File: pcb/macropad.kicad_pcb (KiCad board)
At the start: 2 copper layers, 135 x 79.3 mm, 36 parts, among them J1 Conn_01x02_Pin, SW1 SW_Push, SW10 SW_Push, SW11 SW_Push, SW12 SW_Push, SW13 SW_Push, SW14 SW_Push, SW15 SW_Push, SW16 SW_Push, SW17 SW_DIP_x01, SW18 SW_Push, SW2 SW_Push, SW3 SW_Push, SW4 SW_Push, SW5 SW_Push, SW6 SW_Push, SW7 SW_Push, SW8 SW_Push, SW9 SW_Push, U2 ProMicro

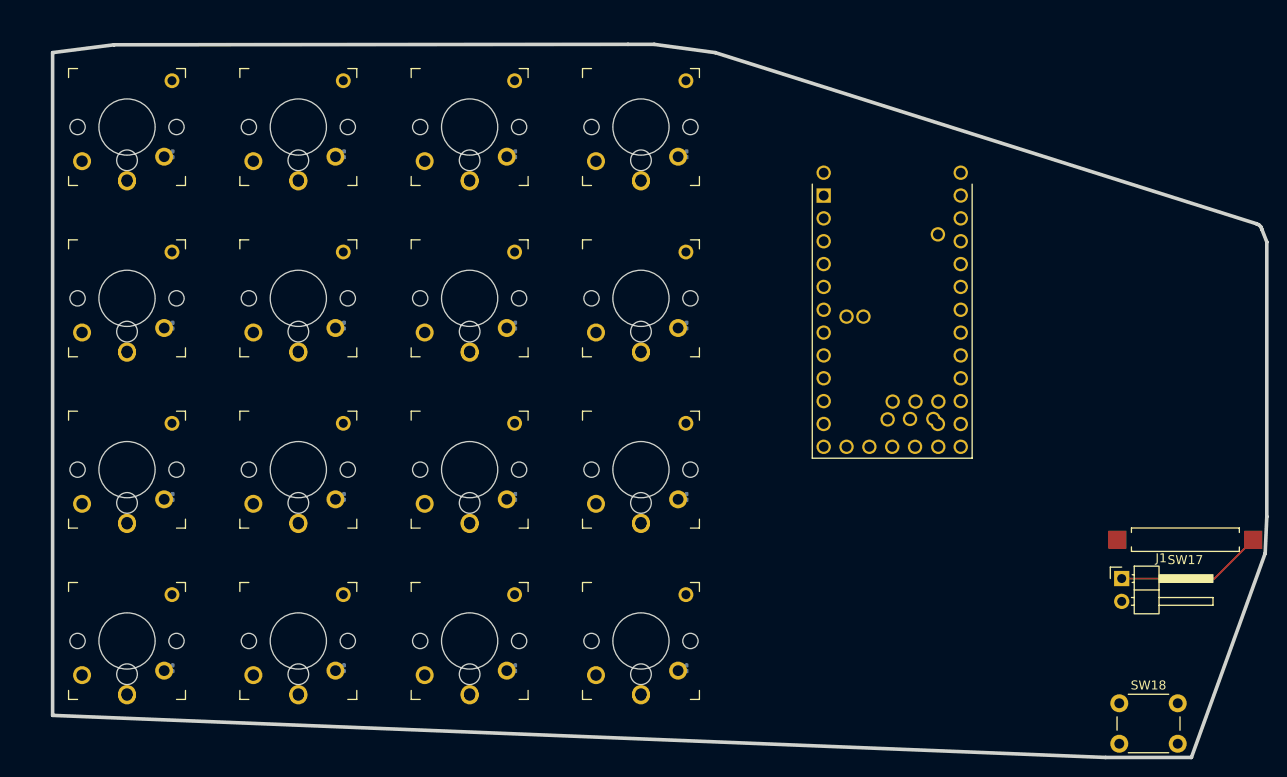
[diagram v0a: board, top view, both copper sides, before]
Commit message: More laying out
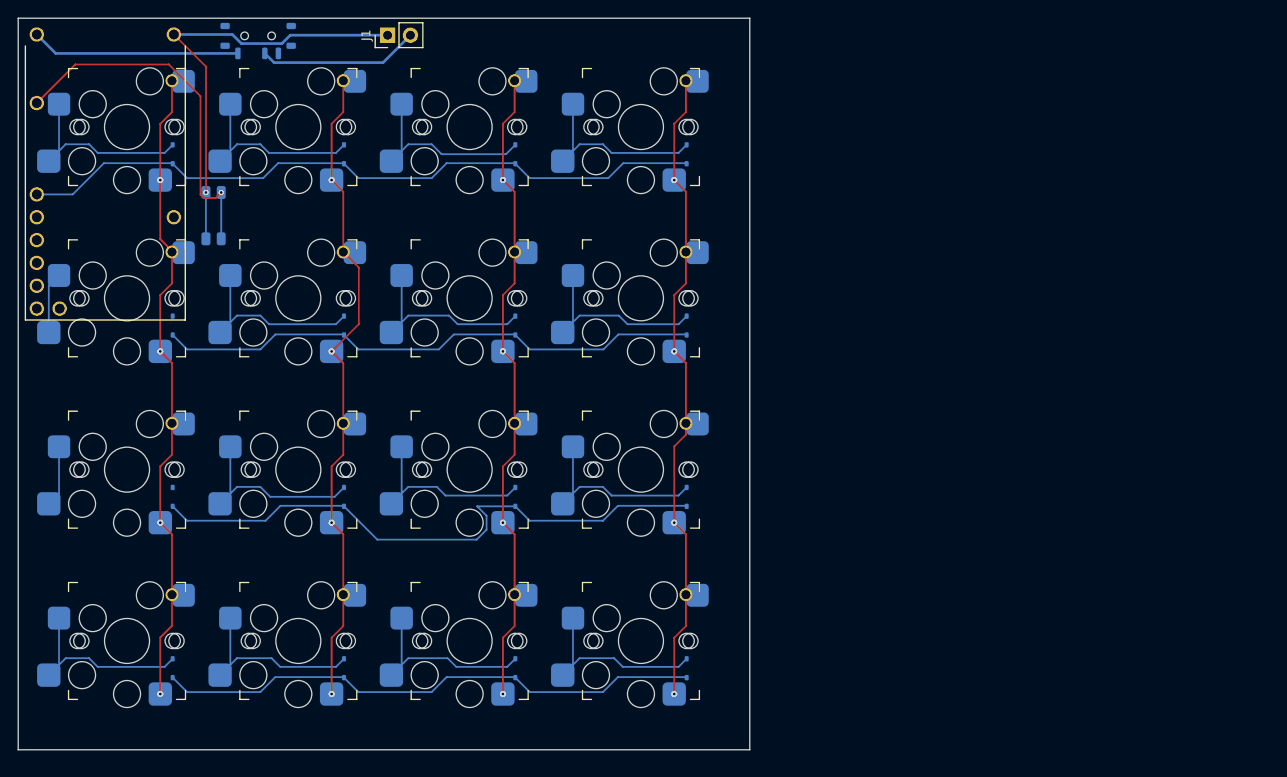
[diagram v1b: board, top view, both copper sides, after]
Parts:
- D1, D10, D11, D12, D13, D14, D15, D16, D2, D3, D4, D5, D6, D7, D8, D9: footprint Diode_SMD:D_0201_0603Metric -> Diode_SMD:D_SOD-323
- J1: footprint Connector_PinHeader_2.54mm:PinHeader_1x02_P2.54mm_Horizontal -> Connector_PinHeader_2.54mm:PinHeader_1x02_P2.54mm_Vertical
- SW1, SW10, SW11, SW12, SW13, SW14, SW15, SW16, SW2, SW3, SW4, SW5, SW6, SW7, SW8, SW9: footprint key-switches:SW_MX_LowProfile_Kailh_Choc_V1V2_THT_Hybrid -> key-switches:SW_MX_Kailh_Choc_V1V2_HotSwap_Hybrid
- SW17: footprint Button_Switch_SMD:SW_SPST_REED_CT10-XXXX-G1 -> Button_Switch_SMD:SW_SPDT_Shouhan_MSK12C02; moved to B.Cu
- SW18: footprint Button_Switch_THT:SW_PUSH_6mm -> Button_Switch_SMD:SW_SPST_EVQP2_MiddlePushTravel_H2.5mm; moved to B.Cu
- U2: footprint TheOneProMicro:TheOneProMicro -> TheOneProMicro:TheOneProMacro
- moved SW17 117.3 mm to (52.7, 28.0)
- moved SW18 114.4 mm to (47.7, 48.0), turned to 90 degrees
- moved J1 101.6 mm to (67.1, 27.9), turned to 90 degrees
- moved U2 88.8 mm to (37.0, 43.1)
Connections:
- SW17 pad 2: Net-(J1-Pin_1) -> Net-(J1-Pin_2)
- SW18 pad 2: Net-(SW18-Pad2) -> Net-(J1-Pin_1)
- U2 pad 13: unconnected-(U2-GP21-Pad13) -> COL1
- U2 pad 14: unconnected-(U2-GP23-Pad14) -> COL0
- U2 pad 30: unconnected-(U2-GP16-Pad30) -> COL3
- U2 pad 33: Net-(J1-Pin_2) -> Net-(J1-Pin_1)
- U2 pad 8: COL1 -> COL2
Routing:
- net ROW0: track 0.00 -> 77.9 mm
- net COL1: track 0.00 -> 73.4 mm, vias 0 -> 4
- net COL0: track 0.00 -> 72.0 mm, vias 0 -> 4
- net COL2: track 0.00 -> 72.0 mm, vias 0 -> 4
- net COL3: track 0.00 -> 72.0 mm, vias 0 -> 4
- net ROW2: track 0.00 -> 66.0 mm
- net ROW1: track 0.00 -> 61.3 mm
- net ROW3: track 0.00 -> 61.3 mm
- net Net-(U2-RST): track 0.00 -> 40.3 mm, vias 0 -> 1
- net Net-(J1-Pin_1): track 16.4 -> 48.8 mm, vias 0 -> 1
- net Net-(U2-GP11(B+)): track 0.00 -> 23.2 mm
- net Net-(D10-A): track 1.19 -> 22.3 mm
- net Net-(D3-A): track 1.19 -> 22.3 mm
- net Net-(D4-A): track 1.19 -> 22.1 mm
- net Net-(D2-A): track 1.19 -> 22.1 mm
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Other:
- board size 135 x 79.3 mm -> 81.3 x 81.3 mm
- board text added: "GP11/B+"
